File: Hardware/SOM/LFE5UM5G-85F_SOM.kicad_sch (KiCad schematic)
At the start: 0 parts

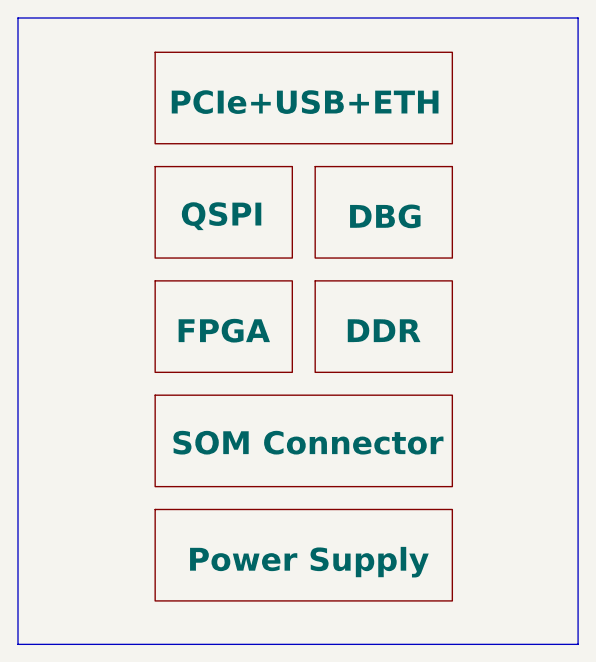
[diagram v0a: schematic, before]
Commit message: SOM: layout update
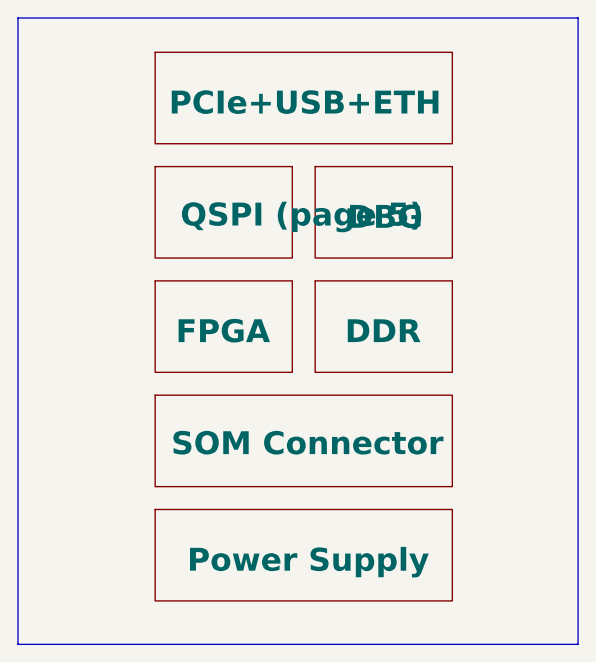
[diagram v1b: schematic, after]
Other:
- sheet QSPI renamed QSPI (page 5)
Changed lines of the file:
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@@
 			(color 0 0 0 0.0000)
 		)
-		(property "Sheetname" "QSPI"
+		(property "Sheetname" "QSPI (page 5)"
 			(at 90.424 104.648 0)
 			(effects
